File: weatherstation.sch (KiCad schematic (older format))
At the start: 20 parts

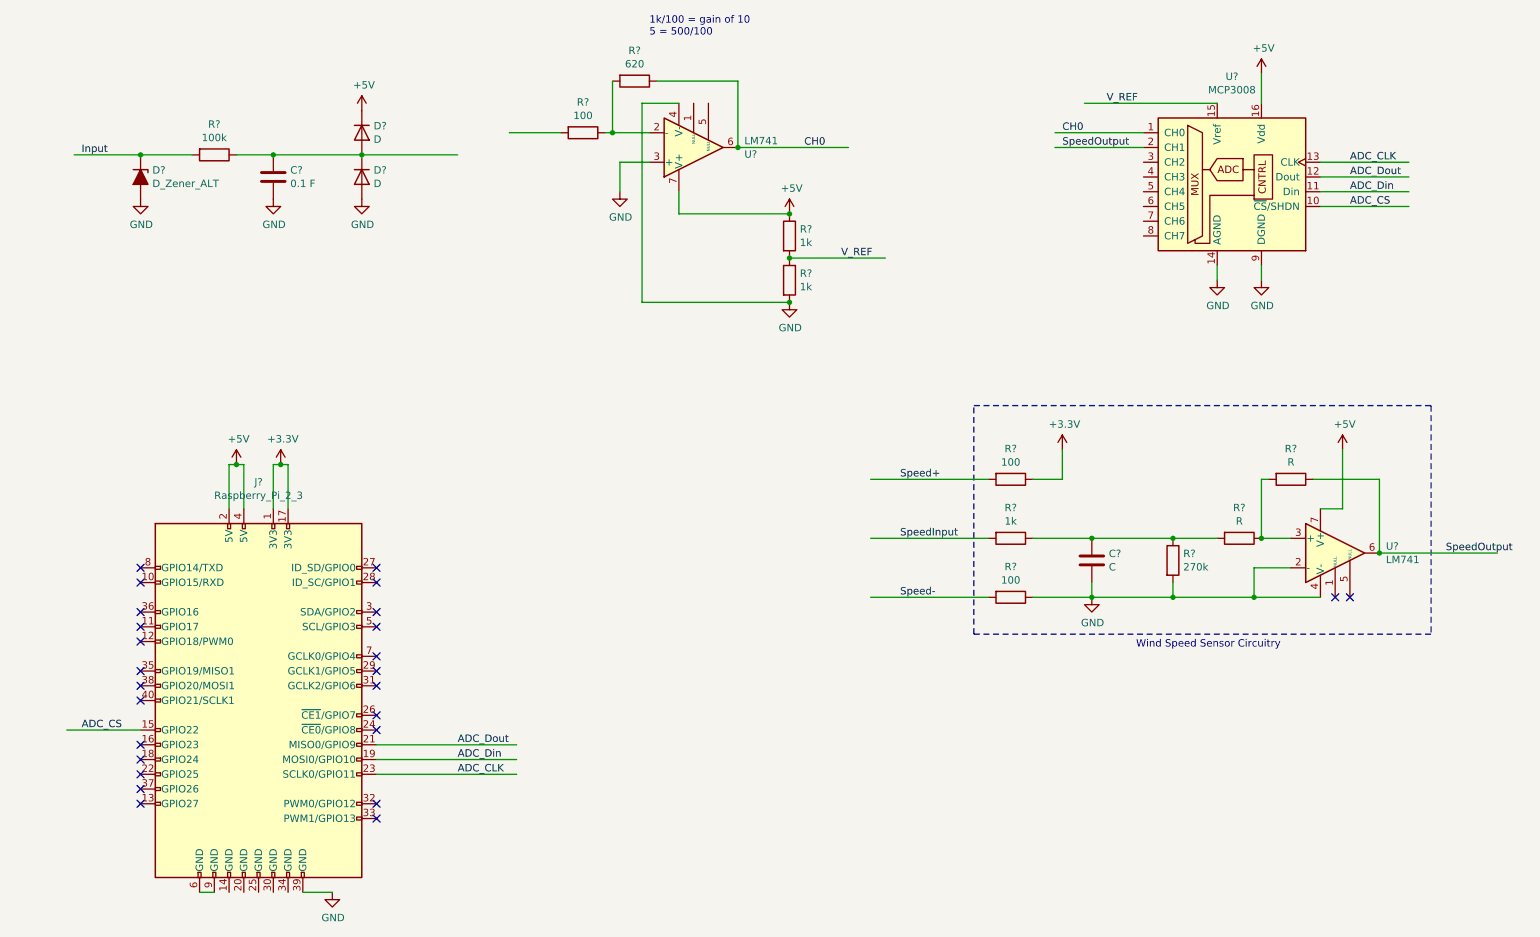
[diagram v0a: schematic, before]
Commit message: Finallized schematic
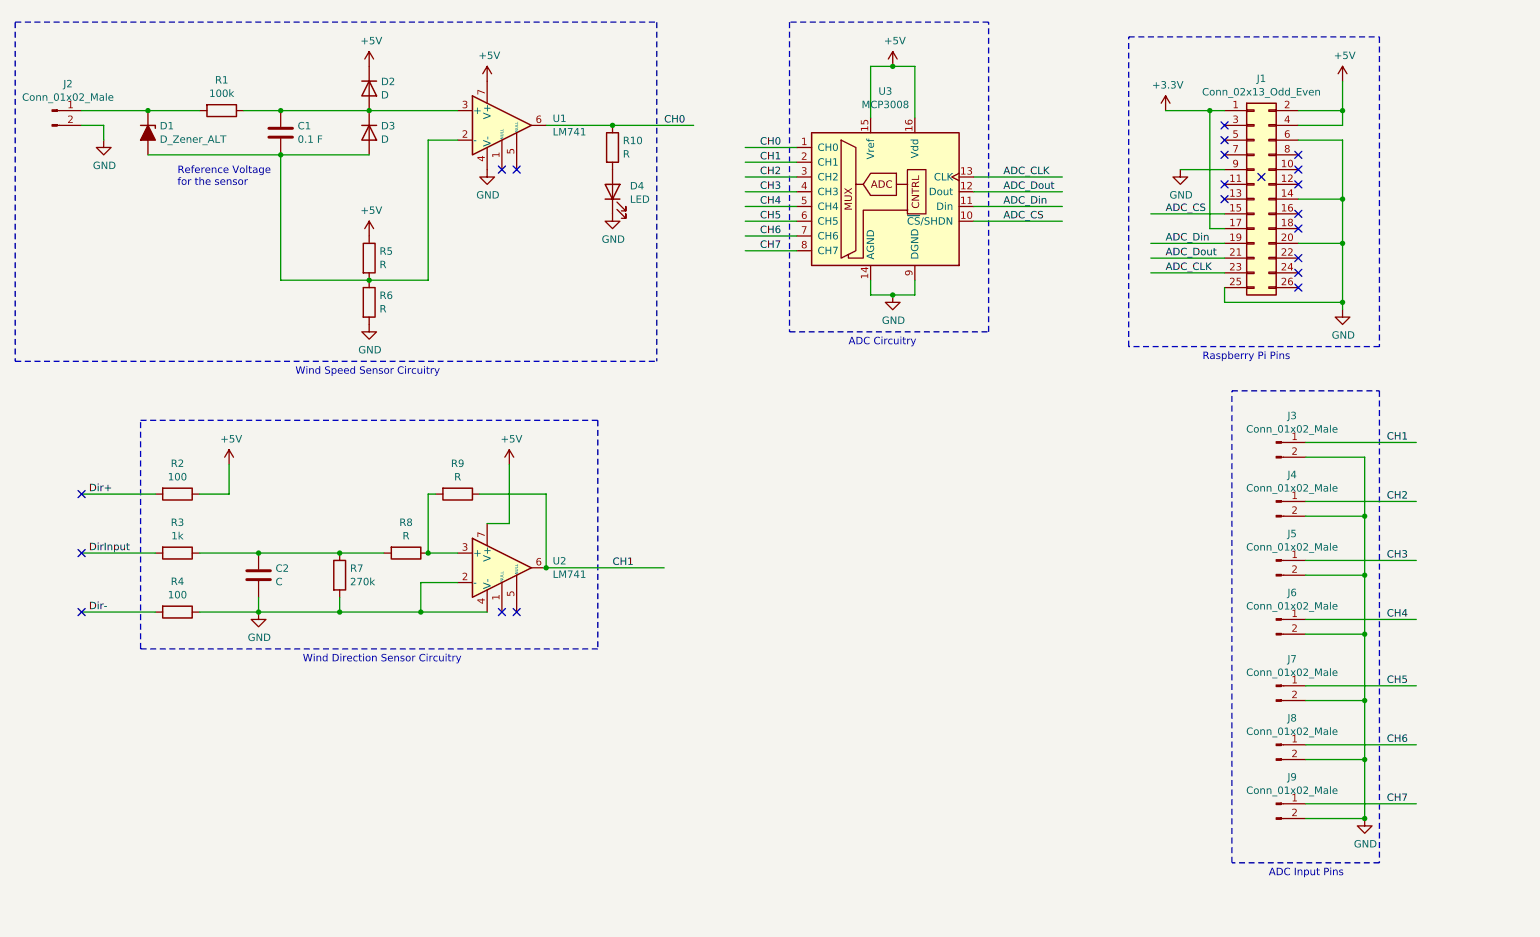
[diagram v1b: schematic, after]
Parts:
- removed J?: Raspberry_Pi_2_3, symbol Connector:Raspberry_Pi_2_3
- removed R?: 620, symbol Device:R
- removed R?: 100, symbol Device:R
- removed R? (x2): 1k, symbol Device:R
- removed U?: LM741, symbol Amplifier_Operational:LM741
- added D4: LED, symbol Device:LED
- added J1: Conn_02x13_Odd_Even, symbol Connector_Generic:Conn_02x13_Odd_Even
- added J2, J3, J4, J5, J6, J7, J8, J9: Conn_01x02_Male, symbol Connector:Conn_01x02_Male
- added R10, R5, R6: R, symbol Device:R
- added U1: LM741, symbol Amplifier_Operational:LM741
- gave numbers to parts that had none: 14
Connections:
- net labels added: CH1, CH2, CH3, CH4, CH5, CH6, CH7, Dir+, Dir-, DirInput
- net labels removed: Input, Speed+, Speed-, SpeedInput, SpeedOutput, V_REF
- wire segments 68 -> 102
- no-connect marks 26 -> 21
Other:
- note added: "ADC Circuitry\n"
- note added: "ADC Input Pins\n"
- note added: "Raspberry Pi Pins\n"
- note added: "Reference Voltage \nfor the sensor\n\n"
- note added: "Wind Direction Sensor Circuitry\n"
- note removed: "1k/100 = gain of 10\n5 = 500/100\n"
- moved on the sheet: C1, C2, D1, D2, D3, R1, R2, R3, R4, R7, R8, R9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
